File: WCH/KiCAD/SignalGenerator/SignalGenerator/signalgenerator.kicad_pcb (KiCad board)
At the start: 2 copper layers, 78.7 x 35.6 mm, 19 parts, among them J1 Conn_01x10, J2 Conn_01x10, J3 Conn_02x05_Odd_Even, J4 Conn_01x02, J5 Conn_01x07_Pin, SW1 UP, SW2 DOWN, SW3 LEFT, SW4 RIGHT, SW5 ENTER, U1 CH32V003F4P6, U2 AMS1117-3.3, Y1 Crystal_GND24_Small

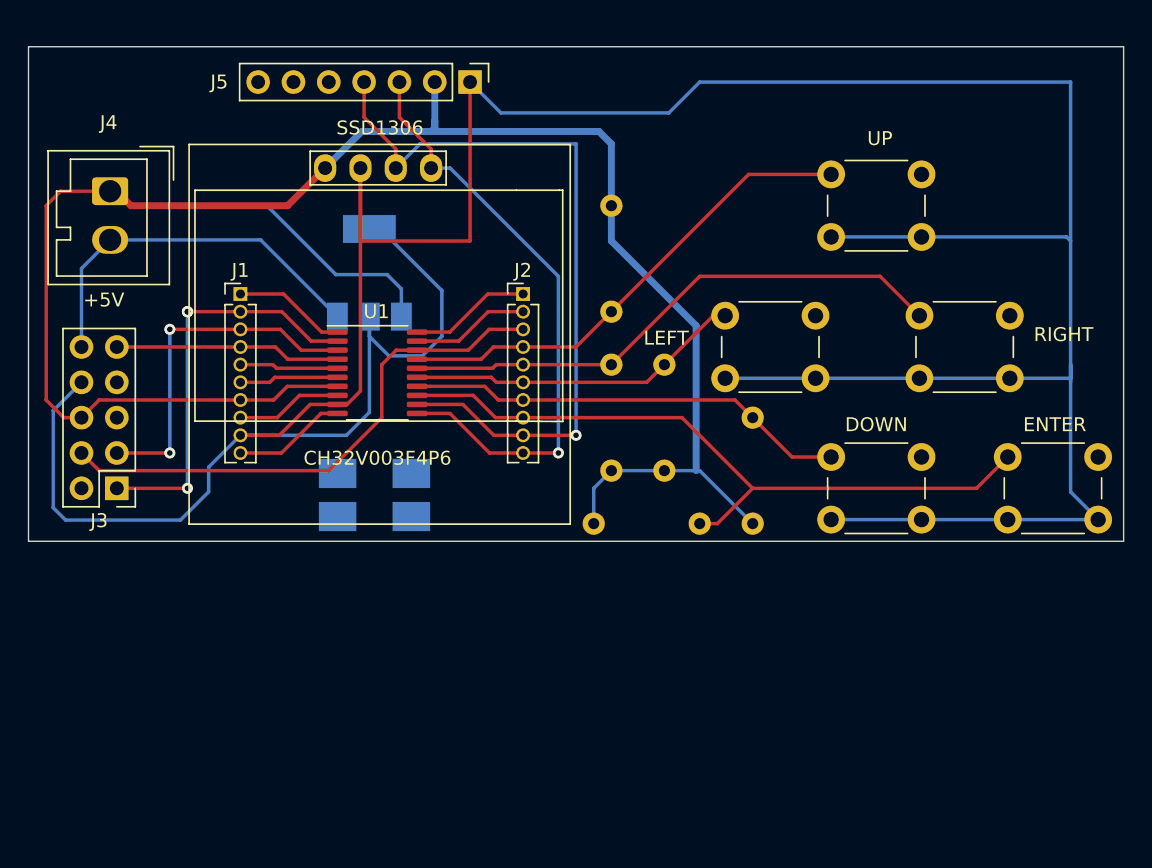
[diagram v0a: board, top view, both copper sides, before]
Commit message: New sigal generator board
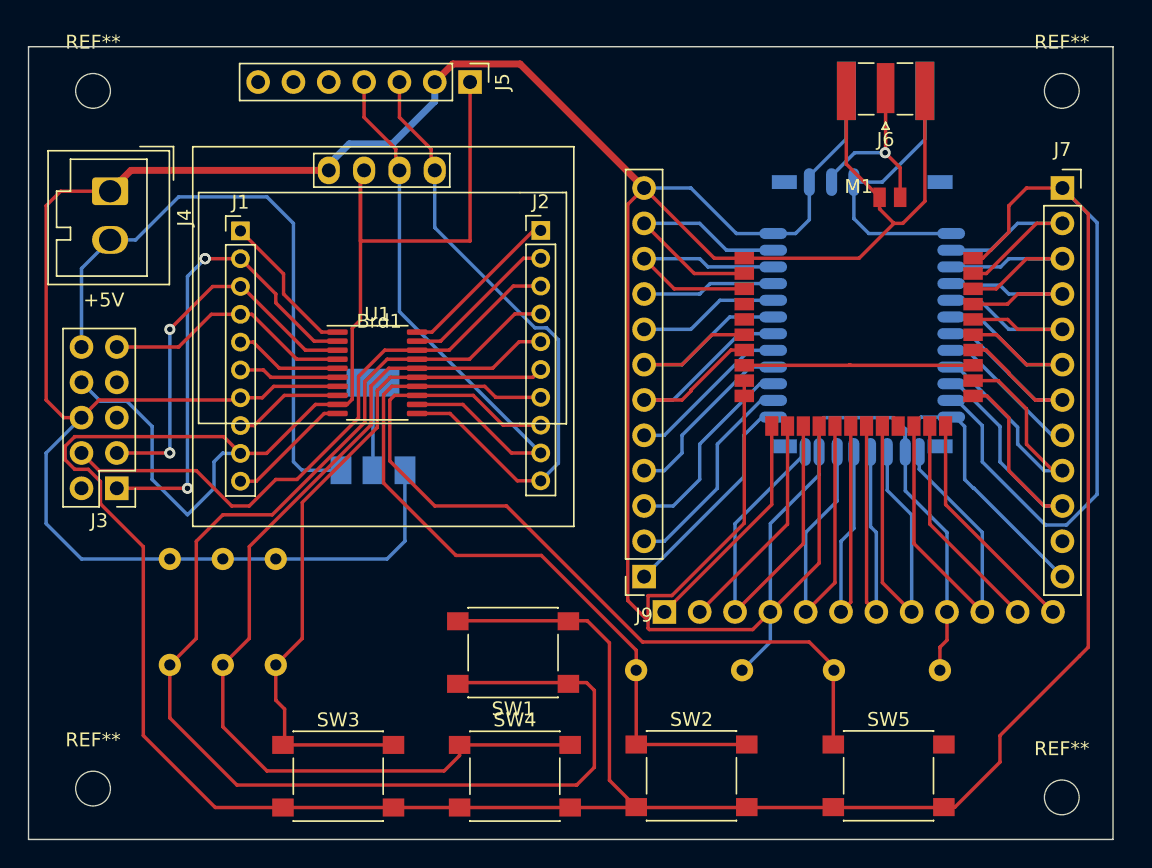
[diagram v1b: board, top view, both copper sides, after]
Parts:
- removed Y1: Crystal_GND24_Small, Crystal:Crystal_SMD_0603-4Pin_6.0x3.5mm_HandSoldering
- added J6: Conn_Coaxial, Connector_Coaxial:SMA_Samtec_SMA-J-P-X-ST-EM1_EdgeMount, F.Cu at (84.5, 26.0)
- added J7: Conn_01x12, Connector_PinSocket_2.54mm:PinSocket_1x12_P2.54mm_Vertical, F.Cu at (97.2, 33.0)
- added J8: Conn_01x12, Connector_PinSocket_2.54mm:PinSocket_1x12_P2.54mm_Vertical, B.Cu at (68.6, 63.5)
- added J9: Conn_01x12, Connector_PinSocket_2.54mm:PinSocket_1x12_P2.54mm_Vertical, F.Cu at (67.1, 61.0)
- added M1: ~, Library:LR1262, F.Cu at (82.5, 41.9)
- added REF**: MountingHole_2.5mm, MountingHole:MountingHole_2.5mm, F.Cu at (97.2, 76.8)
- added REF**: MountingHole_2.5mm, MountingHole:MountingHole_2.5mm, F.Cu at (97.2, 26.0)
- added REF**: MountingHole_2.5mm, MountingHole:MountingHole_2.5mm, F.Cu at (27.5, 76.2)
- added REF**: MountingHole_2.5mm, MountingHole:MountingHole_2.5mm, F.Cu at (27.5, 26.0)
- added U3: RN42N, RF_Module:RN42N, B.Cu at (82.8, 42.3)
- J1, J2: footprint Connector_PinHeader_1.27mm:PinHeader_1x10_P1.27mm_Vertical -> Connector_PinHeader_2.00mm:PinHeader_1x10_P2.00mm_Vertical
- SW1, SW2, SW3, SW4, SW5: footprint Button_Switch_THT:SW_PUSH_6mm -> Button_Switch_SMD:SW_Push_1P1T_NO_6x6mm_H9.5mm
- moved SW4 44.1 mm to (57.8, 75.3)
- moved SW3 43.2 mm to (45.1, 75.3)
- moved SW1 41.3 mm to (57.7, 66.4), turned to 180 degrees
- moved R1 40.7 mm to (33.0, 67.3)
- moved R3 35.3 mm to (40.6, 67.3), turned to 90 degrees
- moved R4 35.3 mm to (36.8, 67.3), turned to 90 degrees
- moved SW2 25.0 mm to (70.5, 75.3)
- moved SW5 24.5 mm to (84.7, 75.3)
- moved R2 20.0 mm to (66.5, 67.7), turned to 0 degrees
- moved R5 14.3 mm to (80.8, 67.7), turned to 0 degrees
- moved U2 11.1 mm to (47.6, 50.2)
- moved J2 4.74 mm to (59.7, 36.1)
- moved J1 4.54 mm to (38.1, 36.1)
- moved Brd1 0.31 mm to (48.1, 42.4)
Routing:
- net GND: track 152.8 -> 322.1 mm
- net /UP: track 35.7 -> 95.2 mm
- net +3.3V: track 258.4 -> 298.3 mm
- net /RIGHT: track 40.0 -> 69.9 mm
- net J8_3: track 0.00 -> 29.0 mm
- net J8_10: track 0.00 -> 28.8 mm
- net J9_5: track 0.00 -> 28.3 mm
- net J8_5: track 0.00 -> 26.7 mm
- net J8_8: track 0.00 -> 26.5 mm
- net J8_6: track 0.00 -> 25.5 mm
- net J8_7: track 0.00 -> 25.3 mm
- net J7_3: track 0.00 -> 25.1 mm
- net /LEFT: track 24.3 -> 49.0 mm
- net /DOWN: track 32.0 -> 56.2 mm
- net J9_12: track 0.00 -> 24.0 mm
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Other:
- board size 78.7 x 35.6 mm -> 78 x 57 mm
